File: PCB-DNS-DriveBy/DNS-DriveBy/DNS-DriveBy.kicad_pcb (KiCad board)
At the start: 2 copper layers, 76 x 40 mm, 24 parts, among them J1 JST 2.0, J2 Conn_01x04, J3 Conn_01x03, Q1 2N3904, Q2 2N3904, SW1 SW_SPST, U1 D1 Mini, U2 NEO-6M

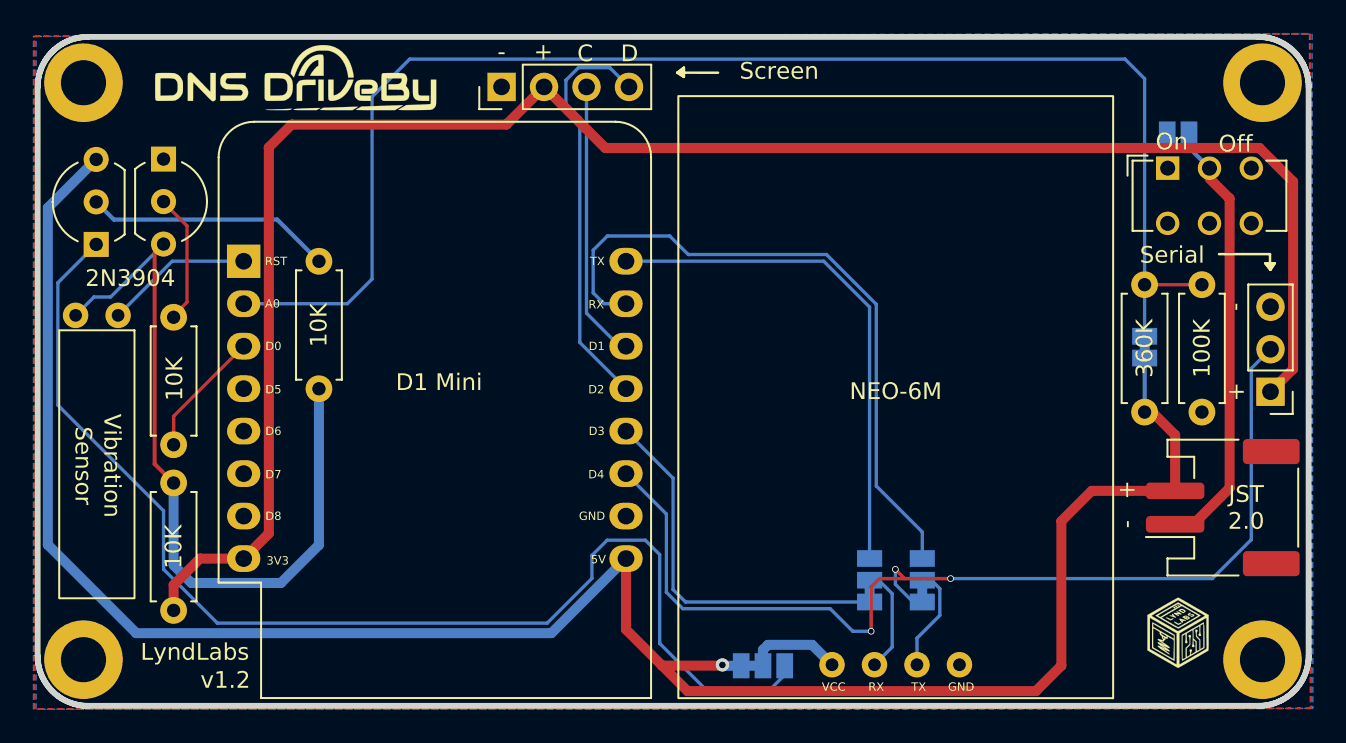
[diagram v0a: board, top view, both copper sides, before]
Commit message: publish v1.3 design files
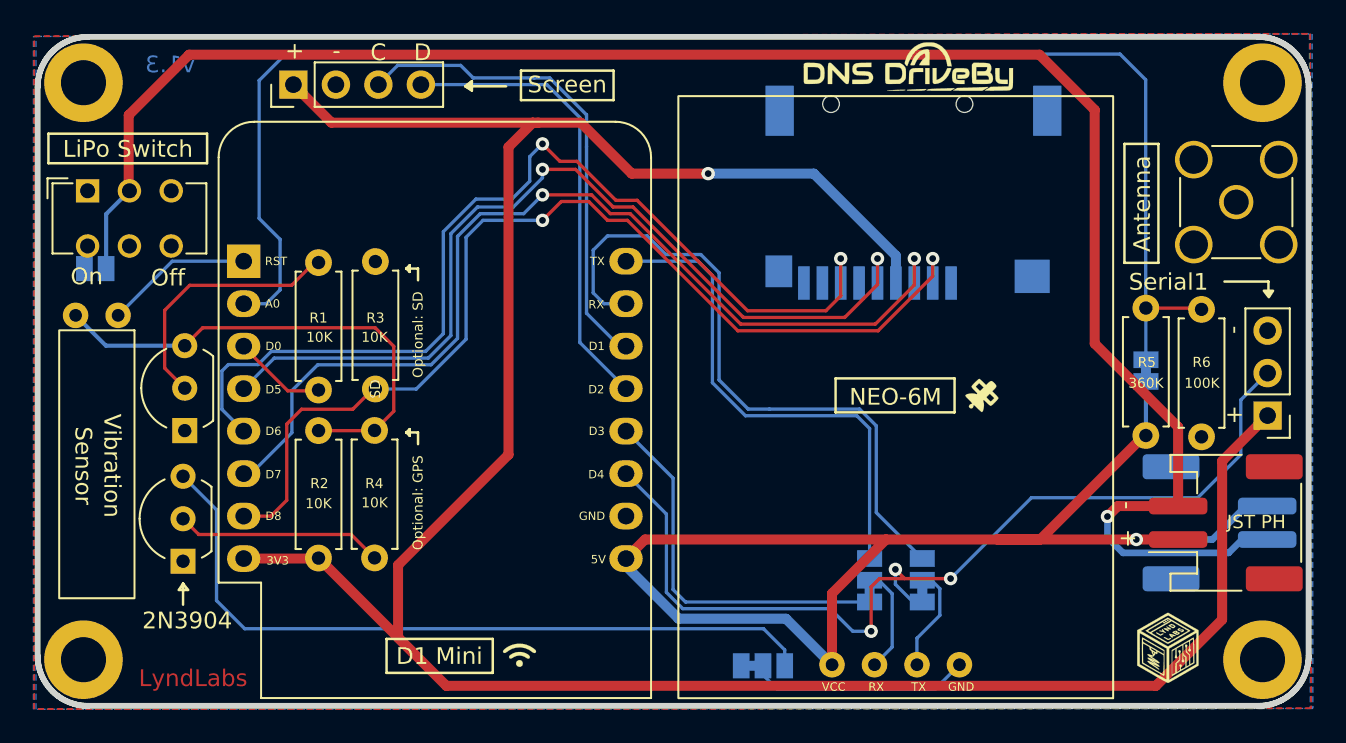
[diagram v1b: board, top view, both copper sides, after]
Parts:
- added Antenna: SMA Antenna, Connector_Coaxial:SMA_Amphenol_901-144_Vertical, F.Cu at (72.4, 10.6)
- added J1: JST 2.0, Connector_JST:JST_PH_S2B-PH-SM4-TB_1x02-1MP_P2.00mm_Horizontal, B.Cu at (71.4, 29.8)
- added J4: Micro_SD_Card_Det, DNS-DriveBy:MicroSD, B.Cu at (53.1, 15.3)
- added R3: 10K, Resistor_THT:R_Axial_DIN0207_L6.3mm_D2.5mm_P7.62mm_Horizontal, F.Cu at (21.0, 21.8)
- J2: value Conn_01x04 -> SH1106
- moved JP5 65.2 mm to (4.21, 14.6)
- moved SW1 64.6 mm to (3.75, 9.96)
- moved Q2 19.6 mm to (9.46, 32.1)
- moved R4 18.0 mm to (20.9, 31.9), turned to 90 degrees
- moved Q1 16.3 mm to (9.56, 24.3), turned to 90 degrees
- moved J2 12.4 mm to (16.1, 3.61)
- moved R1 9.26 mm to (17.6, 21.9)
- moved R2 9.21 mm to (17.6, 24.3)
- moved R6 1.48 mm to (70.4, 17.1)
- moved J3 1.44 mm to (74.3, 23.4)
- moved JP4 1.40 mm to (67.0, 20.7)
- moved R5 1.40 mm to (67.0, 24.6)
- moved Ref** 1.34 mm to (38.8, 21.0)
- moved J1 0.93 mm to (71.8, 29.8)
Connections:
- J1 pad 1: Net-(J1-Pad1) -> +BATT
- J1 pad 2: +BATT -> Net-(J1-Pad2)
- J2 pad 1: GND -> +3V3
- J2 pad 2: +3V3 -> GND
- JP1 pad 1: +BATT -> GND
- JP1 pad 2: Net-(JP1-Pad2) -> Net-(U2-Pad4)
- JP5 pad 2: Net-(J1-Pad1) -> Net-(J1-Pad2)
- Q2 pad 1: Net-(JP1-Pad3) -> GND
- Q2 pad 3: +BATT -> Net-(JP1-Pad3)
- SW1 pad 2: Net-(J1-Pad1) -> Net-(J1-Pad2)
- U2 pad 1: Net-(JP1-Pad2) -> +BATT
- U2 pad 4: GND -> Net-(U2-Pad4)
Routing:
- net Net-(J1-Pad2): track 0.00 -> 111.7 mm, vias 0 -> 1
- net SS: track 0.00 -> 62.2 mm, vias 0 -> 2
- net MISO: track 0.00 -> 59.4 mm, vias 0 -> 2
- net MOSI: track 0.00 -> 59.3 mm, vias 0 -> 2
- net SCK: track 0.00 -> 54.7 mm, vias 0 -> 2
- net +BATT: track 125.4 -> 80.9 mm
- net +3V3: track 109.8 -> 153.9 mm, vias 0 -> 1
- net Net-(JP1-Pad3): track 72.0 -> 45.0 mm
- net Net-(J1-Pad1): track 25.7 -> 0.00 mm
- net GPS-EN: track 46.3 -> 29.5 mm
- net Net-(U2-Pad4): track 0.00 -> 13.3 mm
- net SCL: track 16.7 -> 29.2 mm
- net Net-(Q1-Pad2): track 7.68 -> 15.2 mm
- net Net-(JP1-Pad2): track 5.70 -> 0.00 mm
- net D4: track 63.4 -> 58.6 mm
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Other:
- board text added: "128x64 OLED"
- board text added: "GPS Low-Power"
- board text added: "JST PH"
- board text added: "LiPo Switch"
- board text added: "MicroSD"
- board text added: "Resistor Bypass"
- board text added: "Serial1"
- board text added: "Switch Bypass"
- board text added: "v1.3"
- board text removed: "JST 2.0"
- board text removed: "SSD1306 / SH1106"
- board text removed: "Serial"
- board text removed: "v1.2"
